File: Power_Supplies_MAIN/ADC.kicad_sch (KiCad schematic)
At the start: 35 parts, among them IC1 PCM1865DBT, IC5 PCM1865DBT, J41 PINHD_1x1_Female, J42 PINHD_1x1_Female

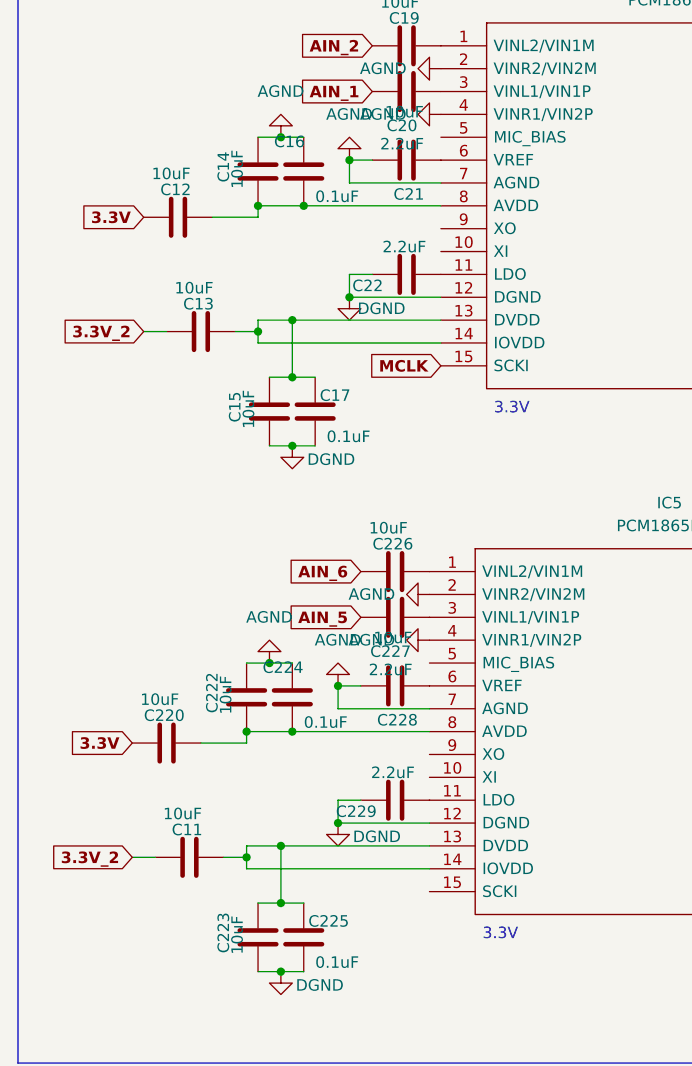
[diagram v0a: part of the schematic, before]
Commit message: added changes that weeks wanted 🐷
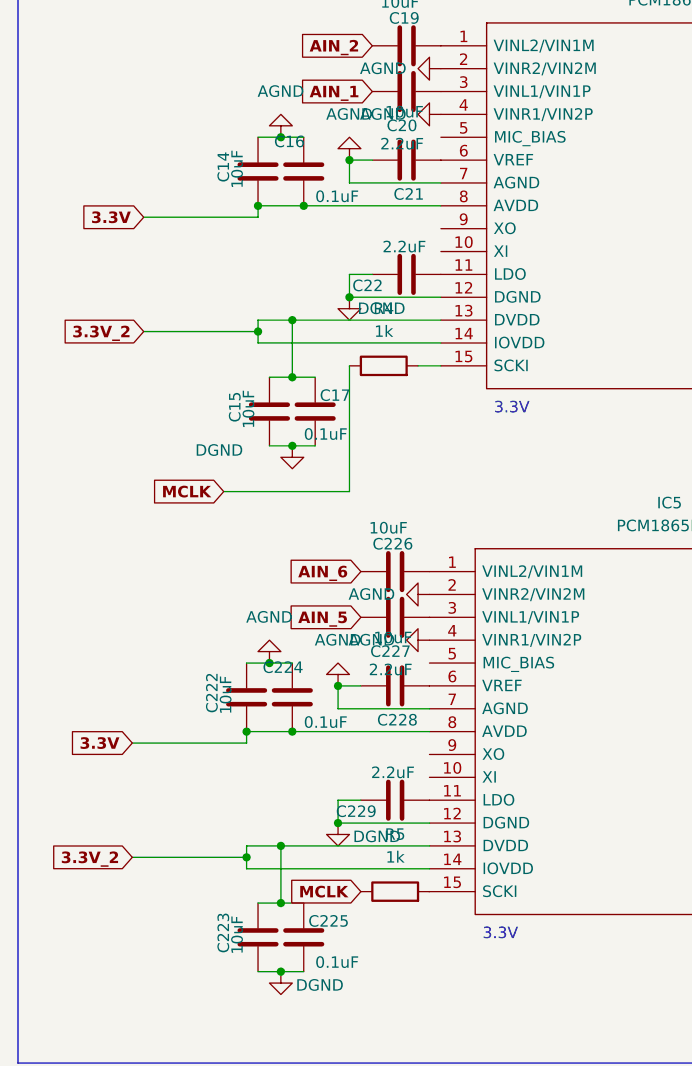
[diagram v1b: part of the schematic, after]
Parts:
- removed C11, C12, C13, C220: 10uF, Capacitor_SMD:C_0805_2012Metric, symbol Device:C
- added R4, R5: 1k, Resistor_SMD:R_0805_2012Metric_Pad1.20x1.40mm_HandSolder, symbol Device:R
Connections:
- net 3.3V: now also C14.2, C16.2, C222.2, C224.2, IC1.8 (AVDD), IC5.8 (AVDD)
- net 3.3V_2: now also C15.1, C17.1, C223.1, C225.1, IC1.13 (DVDD), IC1.14 (IOVDD), IC5.13 (DVDD), IC5.14 (IOVDD)
- net MCLK: now also R4.1, R5.1; no longer IC1.15 (SCKI)
- net at IC5.15 (SCKI): now also R5.2
- new net: IC1.15 (SCKI), R4.2

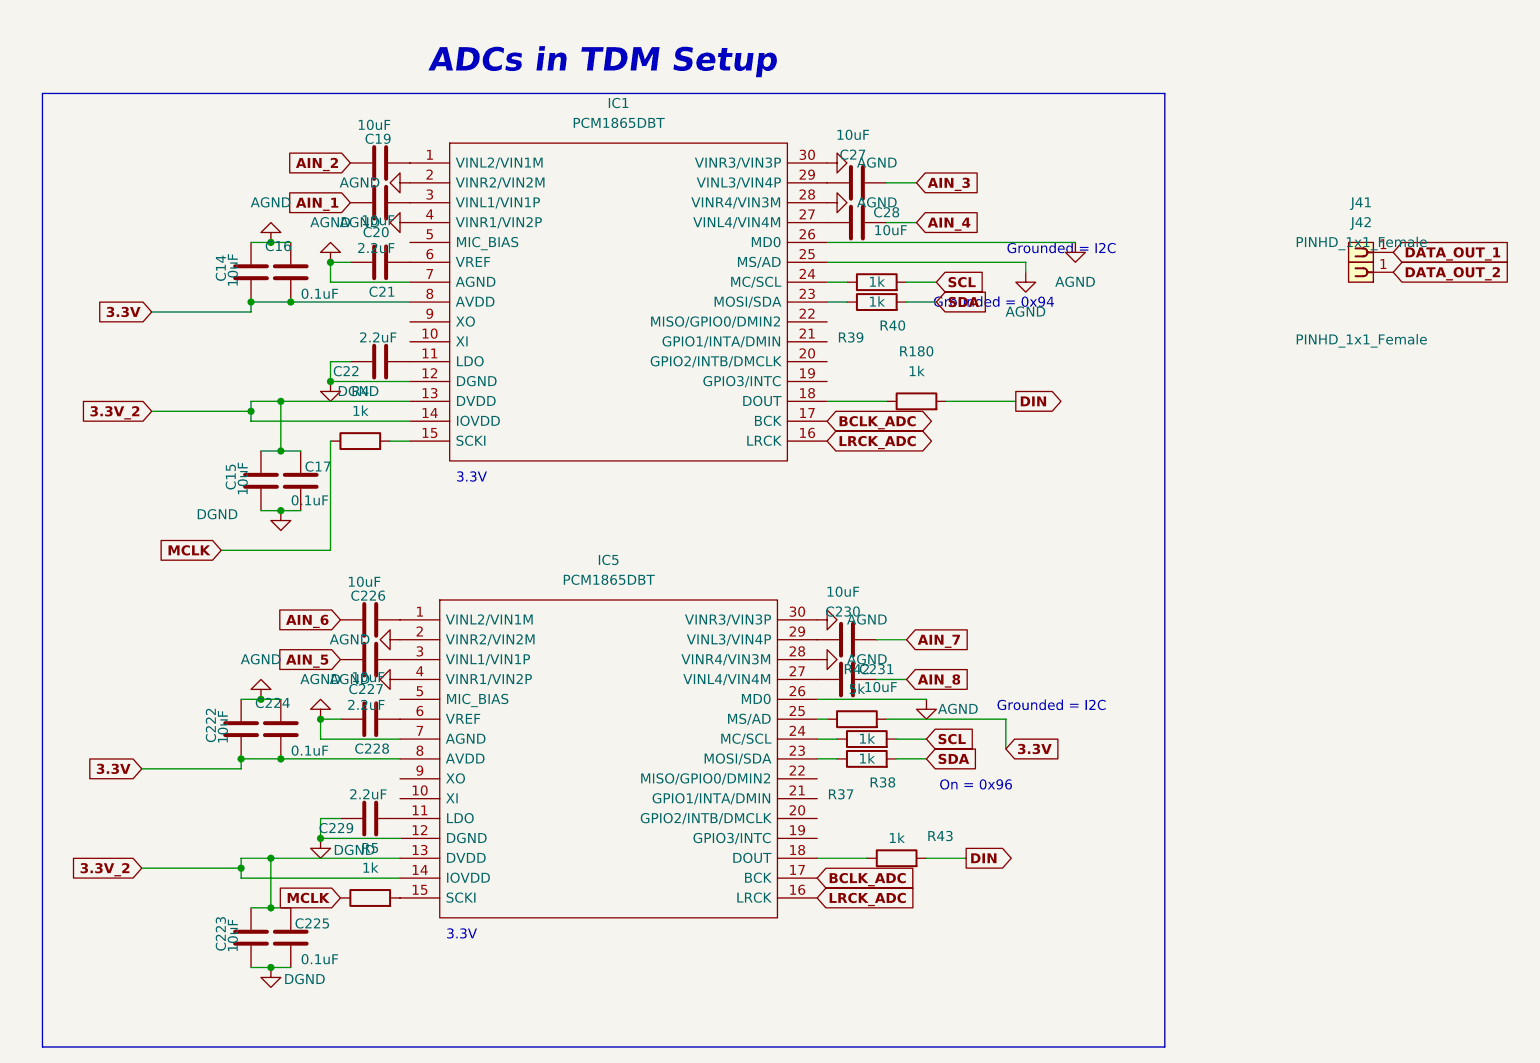
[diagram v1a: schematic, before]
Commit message: fixed a lot of stuff
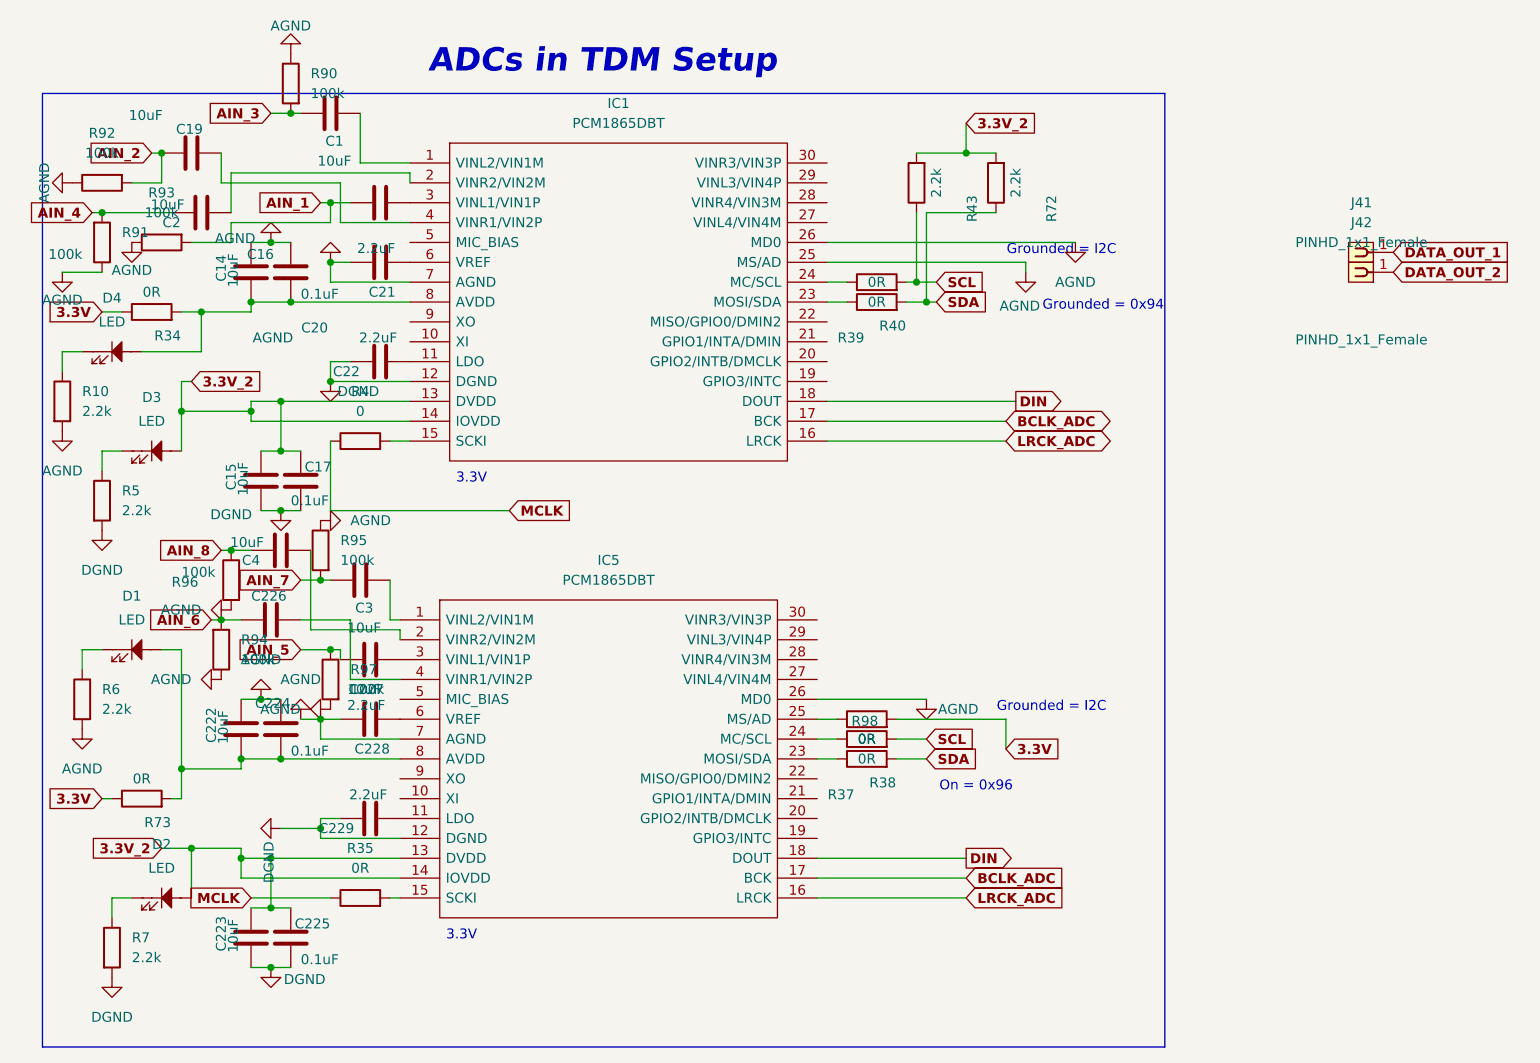
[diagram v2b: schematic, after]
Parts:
- removed C230, C231, C27, C28: 10uF, Capacitor_SMD:C_0805_2012Metric, symbol Device:C
- removed R180: 1k, Resistor_SMD:R_0805_2012Metric_Pad1.20x1.40mm_HandSolder, symbol Device:R
- removed R42: 5k, Resistor_SMD:R_0603_1608Metric_Pad0.98x0.95mm_HandSolder, symbol Device:R
- added C1, C2, C3, C4: 10uF, Capacitor_SMD:C_0805_2012Metric, symbol Device:C
- added D1, D2, D3, D4: LED, LED_SMD:LED_0402_1005Metric_Pad0.77x0.64mm_HandSolder, symbol PCM_SL_Devices:LED
- added R10, R6, R7: 2.2k, Resistor_SMD:R_0805_2012Metric, symbol Device:R
- added R34, R35, R73, R98: 0R, Resistor_SMD:R_0805_2012Metric_Pad1.20x1.40mm_HandSolder, symbol Device:R
- added R72: 2.2k, Resistor_SMD:R_0805_2012Metric_Pad1.20x1.40mm_HandSolder, symbol Device:R
- added R90, R91, R92, R93, R94, R95, R96, R97: 100k, PCM_Resistor_SMD_AKL:R_0402_1005Metric, symbol PCM_Resistor_AKL:R_0402
- R37, R38, R39, R40: value 1k -> 0R
- R4: value 1k -> 0
- R43: value 1k -> 2.2k
- R5: value 1k -> 2.2k; footprint Resistor_SMD:R_0805_2012Metric_Pad1.20x1.40mm_HandSolder -> Resistor_SMD:R_0805_2012Metric
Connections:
- net 3.3V: now also R34.1, R73.1, R98.2; no longer C14.2, C16.2, C222.2, C224.2, IC1.8 (AVDD), IC5.8 (AVDD)
- net 3.3V_2: now also R43.2, D2.2, D3.2, R72.2
- net AGND: now also R10.2, R6.2, R90.2, R91.2, R92.2, R93.2, R94.2, R95.2, R96.1, R97.1; no longer IC1.2 (VINR2/VIN2M), IC1.28 (VINR4/VIN3M), IC1.30 (VINR3/VIN3P), IC1.4 (VINR1/VIN2P), IC5.2 (VINR2/VIN2M), IC5.28 (VINR4/VIN3M), IC5.30 (VINR3/VIN3P), IC5.4 (VINR1/VIN2P)
- net AIN_1: now also R93.1
- net AIN_2: now also R92.1
- net AIN_3: now also C1.2, R90.1
- net AIN_4: now also C2.2, R91.1
- net AIN_5: now also R97.2
- net AIN_6: now also R94.1
- net AIN_7: now also C3.2, R95.1
- net AIN_8: now also C4.2, R96.2
- net DGND: now also R5.2, R7.2
- net DIN: now also IC1.18 (DOUT), IC5.18 (DOUT); no longer R43.2
- net MCLK: now also R35.1; no longer R5.1
- net SCL: now also R43.1
- net SDA: now also R72.1
- net at IC5.15 (SCKI): now also R35.2; no longer R5.2
- net at C19.2: now also IC1.4 (VINR1/VIN2P); no longer IC1.1 (VINL2/VIN1M)
- net at IC5.1 (VINL2/VIN1M): now also C3.1; no longer C226.2
- net at IC5.25 (MS/AD): now also R98.1
- new net: C14.2, C16.2, D4.2, IC1.8 (AVDD), R34.2
- new net: D2.1, R7.1
- new net: C2.1, IC1.2 (VINR2/VIN2M)
- new net: D1.1, R6.1
- new net: C222.2, C224.2, D1.2, IC5.8 (AVDD), R73.2
- new net: C4.1, IC5.2 (VINR2/VIN2M)
- new net: C226.2, IC5.4 (VINR1/VIN2P)
- new net: C1.1, IC1.1 (VINL2/VIN1M)
- new net: D3.1, R5.1
- new net: D4.1, R10.1
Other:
- moved on the sheet: C19, C226
